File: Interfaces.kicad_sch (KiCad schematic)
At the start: 20 parts, among them J1 I/O_HDR, J2 UART1_HDR, J3 SWDB, J7 I2C2_Headers, J9 I2C1_Headers

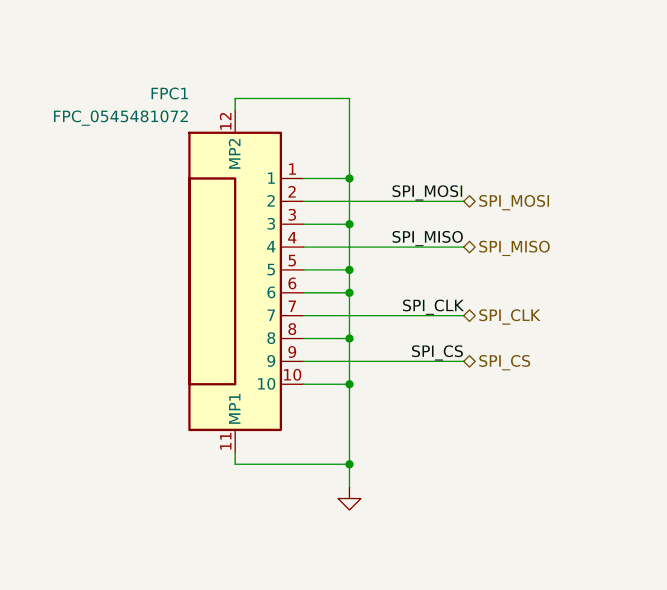
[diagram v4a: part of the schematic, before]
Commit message: Update
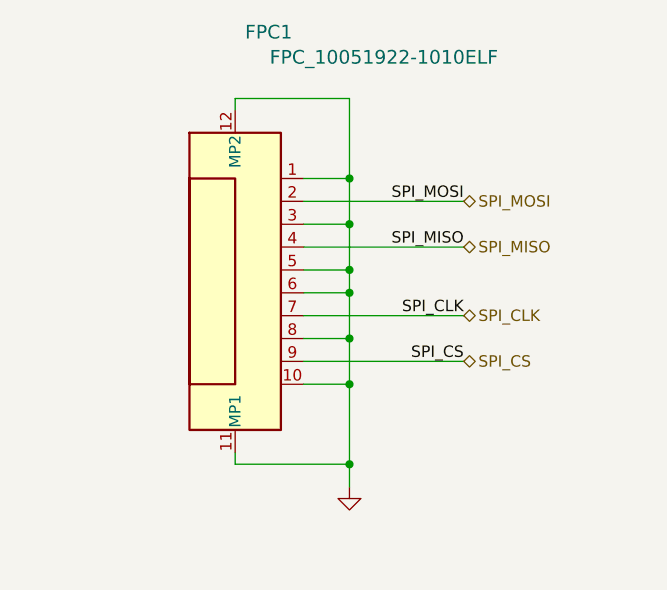
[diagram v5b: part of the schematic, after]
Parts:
- removed FPC1: FPC_0545481072, Personal_Project:FPC_0545481072, symbol Personal_Projects:FPC_0545481072
- added FPC1: FPC_10051922-1010ELF, Personal_Project:FPC_10051922_1010, symbol Personal_Projects:FPC_10051922-1010ELF
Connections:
- net GND: now also FPC1.1, FPC1.10, FPC1.11 (MP1), FPC1.12 (MP2), FPC1.3, FPC1.5, FPC1.6, FPC1.8
- net SPI_CLK: now also FPC1.7
- net SPI_CS: now also FPC1.9
- net SPI_MISO: now also FPC1.4
- net SPI_MOSI: now also FPC1.2
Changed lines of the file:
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@@
 	)
 	(symbol
-		(lib_id "Personal_Projects:FPC_0545481072")
+		(lib_id "Personal_Projects:FPC_10051922-1010ELF")
 		(at 43.18 43.18 0)
 		(unit 1)
@@
 		(dnp no)
 		(property "Reference" "FPC1"
-			(at 43.18 33.782 0)
+			(at 54.61 26.924 0)
 			(effects
 				(font
-					(size 1.27 1.27)
+					(size 1.524 1.524)
 				)
 				(justify right)
 			)
 		)
-		(property "Value" "FPC_0545481072"
-			(at 43.18 36.322 0)
+		(property "Value" "FPC_10051922-1010ELF"
+			(at 77.47 29.718 0)
 			(effects
 				(font
-					(size 1.27 1.27)
+					(size 1.524 1.524)
 				)
 				(justify right)
 			)
 		)
-		(property "Footprint" "Personal_Project:FPC_0545481072"
-			(at 64.77 138.1 0)
+		(property "Footprint" "Personal_Project:FPC_10051922_1010"
+			(at 43.18 90.17 0)
 			(effects
 				(font
 					(size 1.27 1.27)
+					(italic yes)
 				)
-				(justify left top)
 				(hide yes)
 			)
 		)
-		(property "Datasheet" "https://www.molex.com/en-us/products/part-detail-pdf/545481072?display=pdf"
-			(at 64.77 238.1 0)
+		(property "Datasheet" "10051922-1010ELF"
+			(at 43.18 86.36 0)
 			(effects
 				(font
 					(size 1.27 1.27)
+					(italic yes)
 				)
-				(justify left top)
 				(hide yes)
 			)
 		)
-		(property "Description" "0.50mm Pitch Easy-On FFC/FPC Connector, 1.20mm Height, Right-Angle, Surface Mount, ZIF, Bottom Contact Style, 10 Circuits, Gold (Au) Plating"
-			(at 43.18 73.66 0)
+		(property "Description" ""
+			(at 55.88 43.18 0)
 			(effects
 				(font
@@
 			)
 		)
-		(property "Height" "1.3"
-			(at 64.77 438.1 0)
-			(effects
-				(font
-					(size 1.27 1.27)
-				)
-				(justify left top)
-				(hide yes)
-			)
+		(pin "6"
 		)
-		(property "Arrow Part Number" "0545481072"
-			(at 64.77 538.1 0)
-			(effects
-				(font
-					(size 1.27 1.27)
-				)
-				(justify left top)
-				(hide yes)
-			)
-		)
-		(property "Arrow Price/Stock" ""
-			(at 64.77 638.1 0)
-			(effects
-				(font
-					(size 1.27 1.27)
-				)
-				(justify left top)
-				(hide yes)
-			)
-		)
-		(property "Manufacturer_Name" "Molex"
-			(at 64.77 738.1 0)
-			(effects
-				(font
-					(size 1.27 1.27)
-				)
-				(justify left top)
-				(hide yes)
-			)
-		)
-		(property "Manufacturer_Part_Number" "0545481072"
-			(at 64.77 838.1 0)
-			(effects
-				(font
-					(size 1.27 1.27)
-				)
-				(justify left top)
-				(hide yes)
-			)
+		(pin "9"
 		)
 		(pin "4"
@@
 		(pin "7"
 		)
-		(pin "6"
+		(pin "2"
 		)
 		(pin "5"
 		)
-		(pin "2"
+		(pin "3"
 		)
 		(pin "8"
 		)
-		(pin "3"
+		(pin "12"
 		)
 		(pin "10"
 		)
-		(pin "12"
+		(pin "1"
 		)
 		(pin "11"
 		)
-		(pin "9"
-		)
-		(pin "1"
-		)
 		(instances
-			(project "LoRa_Board"
+			(project ""
 				(path "/34ccaf76-212c-4f8e-9afa-bb7eea5015e3/336ebea6-c9a7-4c8d-a774-b509fb11d0ab"
 					(reference "FPC1")

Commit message: Update Readme file
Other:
- company: (none) -> Peter Hancak
- title: (none) -> LoRa Board
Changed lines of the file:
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@@
 	(generator_version "8.0")
 	(paper "USLetter")
+	(title_block
+		(title "LoRa Board")
+		(date "2026-03-17")
+		(rev "B")
+		(company "Peter Hancak")
+	)
 	(junction
 		(at 217.17 121.92)

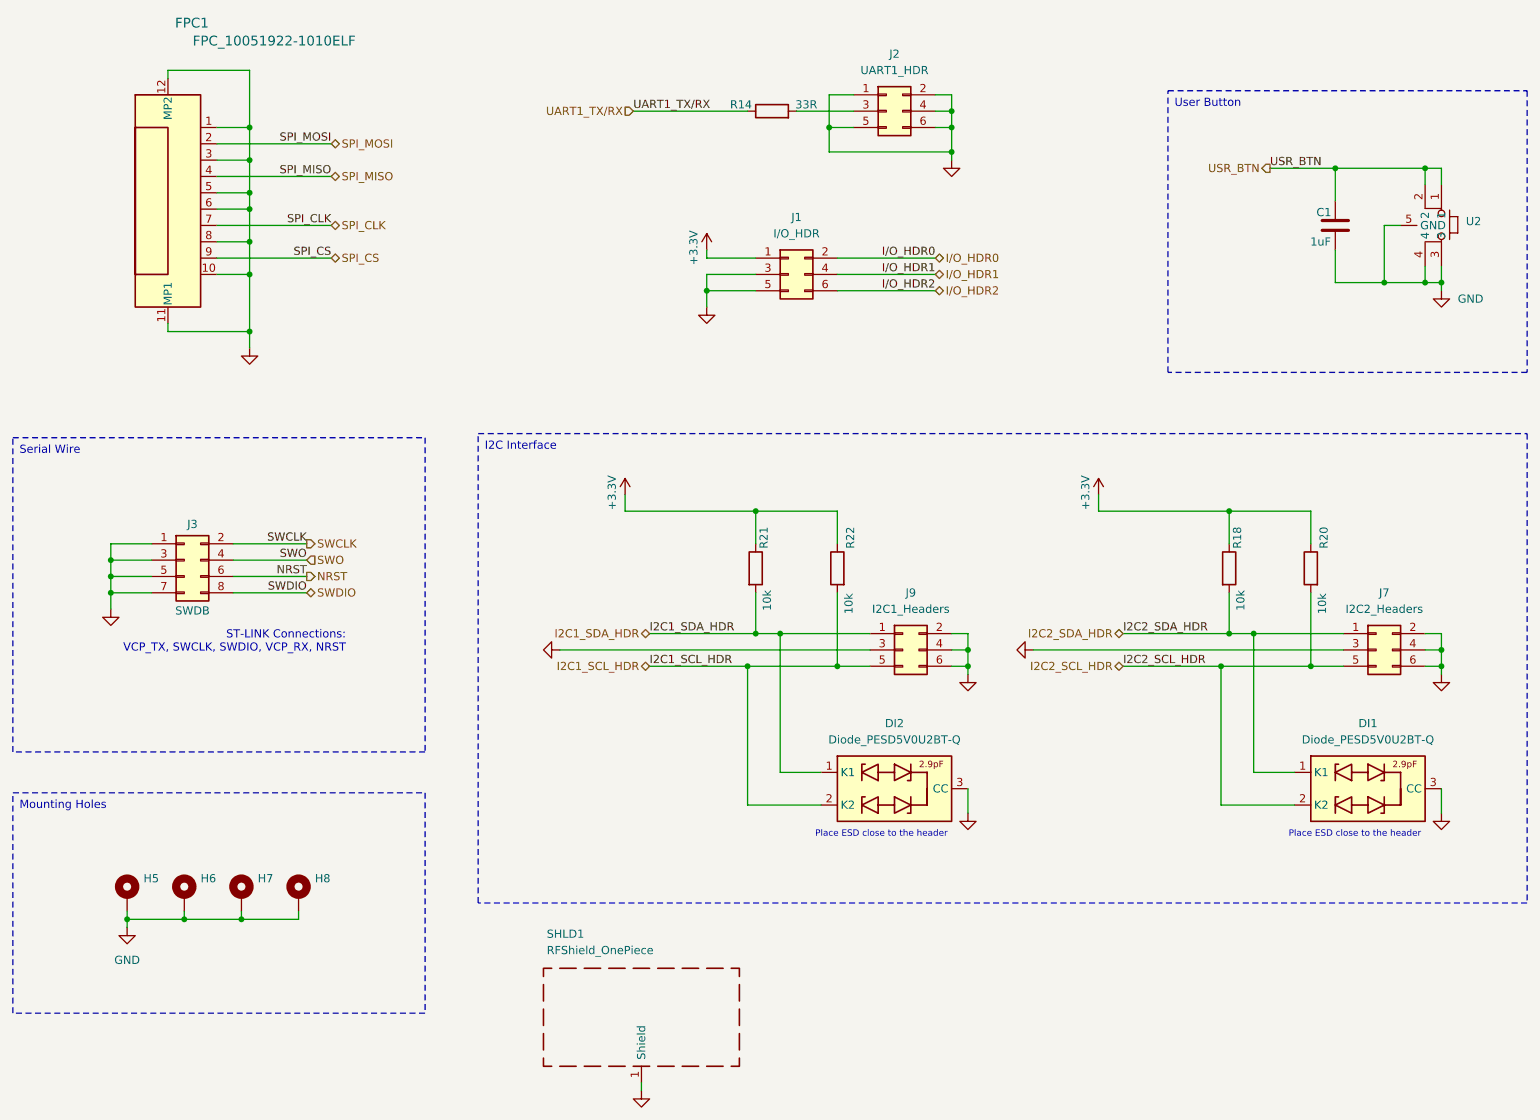
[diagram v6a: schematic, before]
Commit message: Update
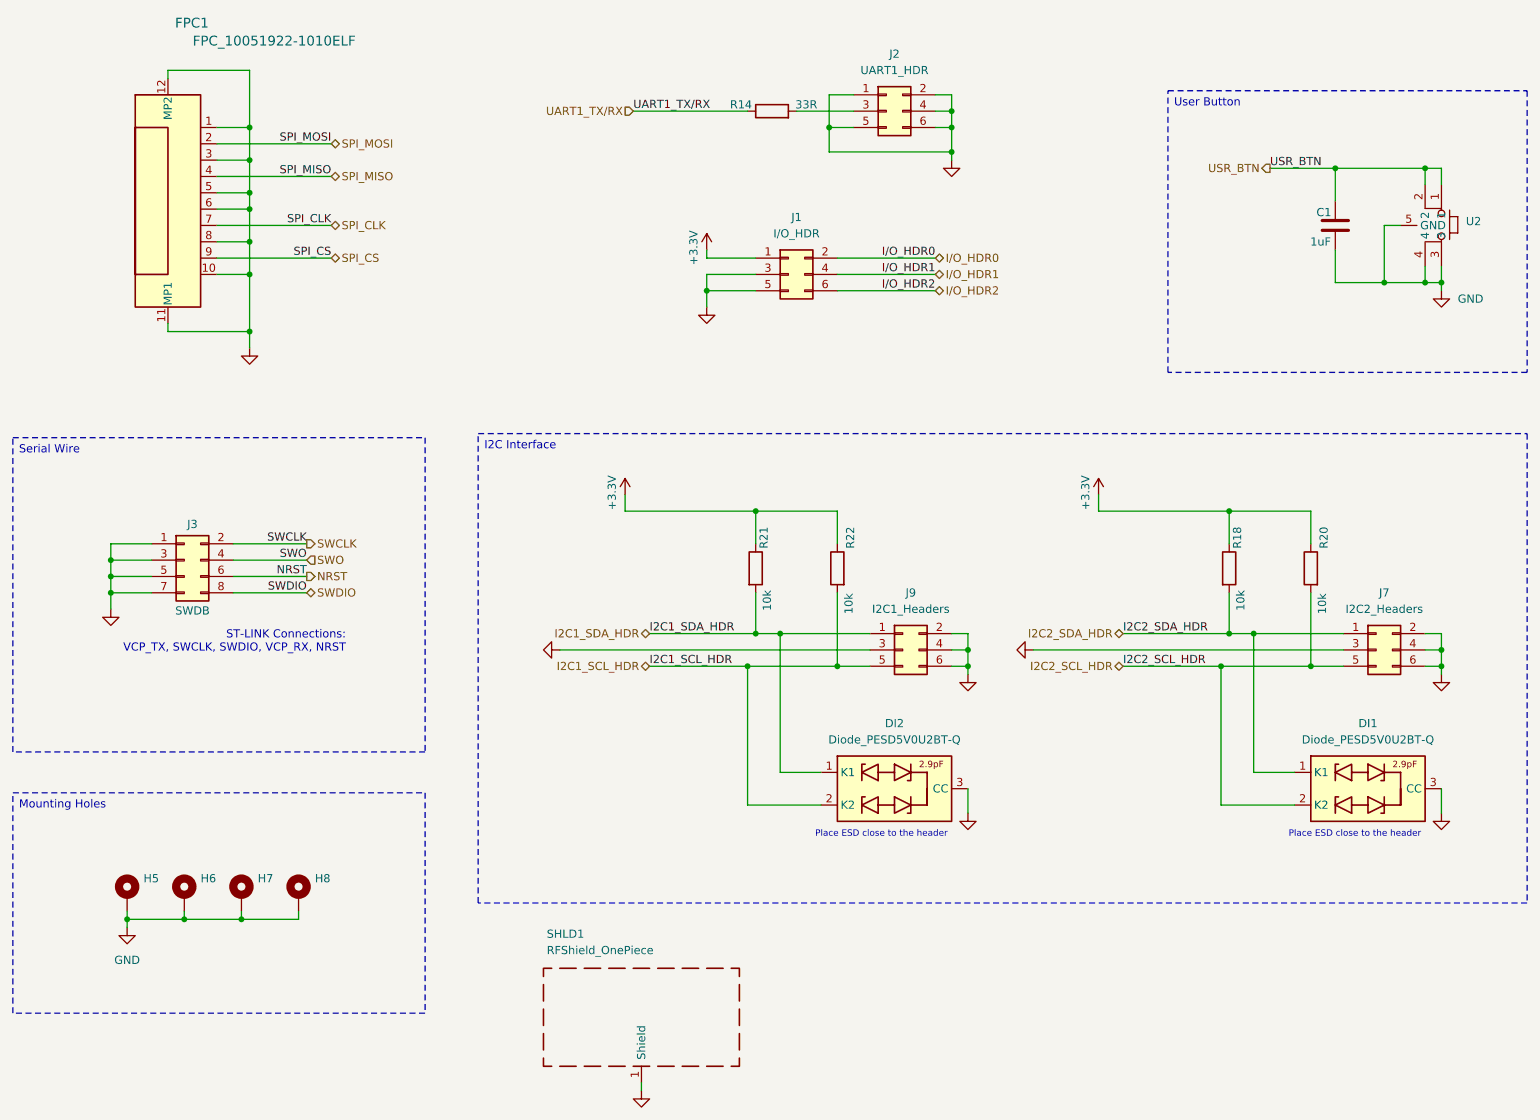
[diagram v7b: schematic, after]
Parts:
- U2: value ~ -> (none)
